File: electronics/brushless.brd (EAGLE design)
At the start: 35.5 x 43.3 mm, 69 parts, among them J1 USB_MINI-B_SMT, Q1 BUK7Y12-40E, Q2 BUK7Y12-40E, Q3 BUK7Y12-40E, Q4 BUK7Y12-40E, Q5 BUK7Y12-40E, Q6 BUK7Y12-40E, X1 JST-XH-10-PIN-LONG-PAD

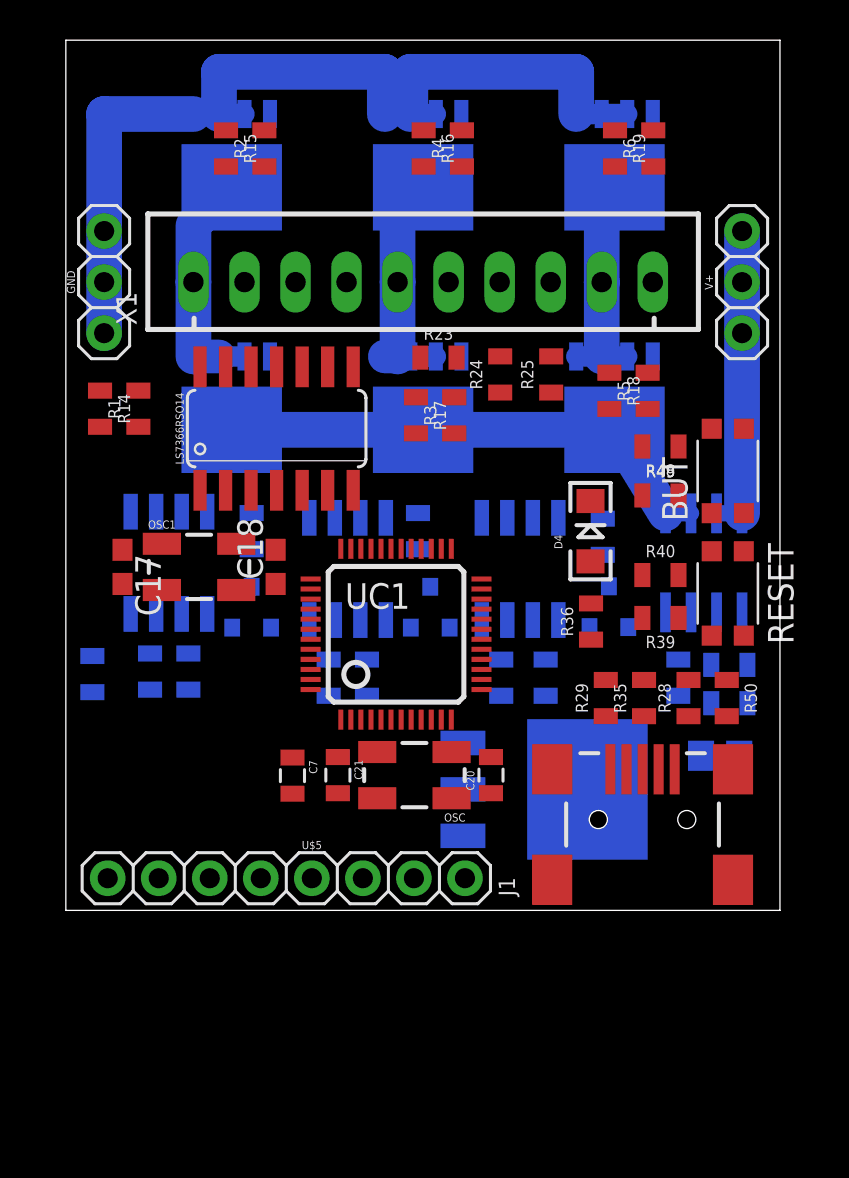
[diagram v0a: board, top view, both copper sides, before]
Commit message: Controller board
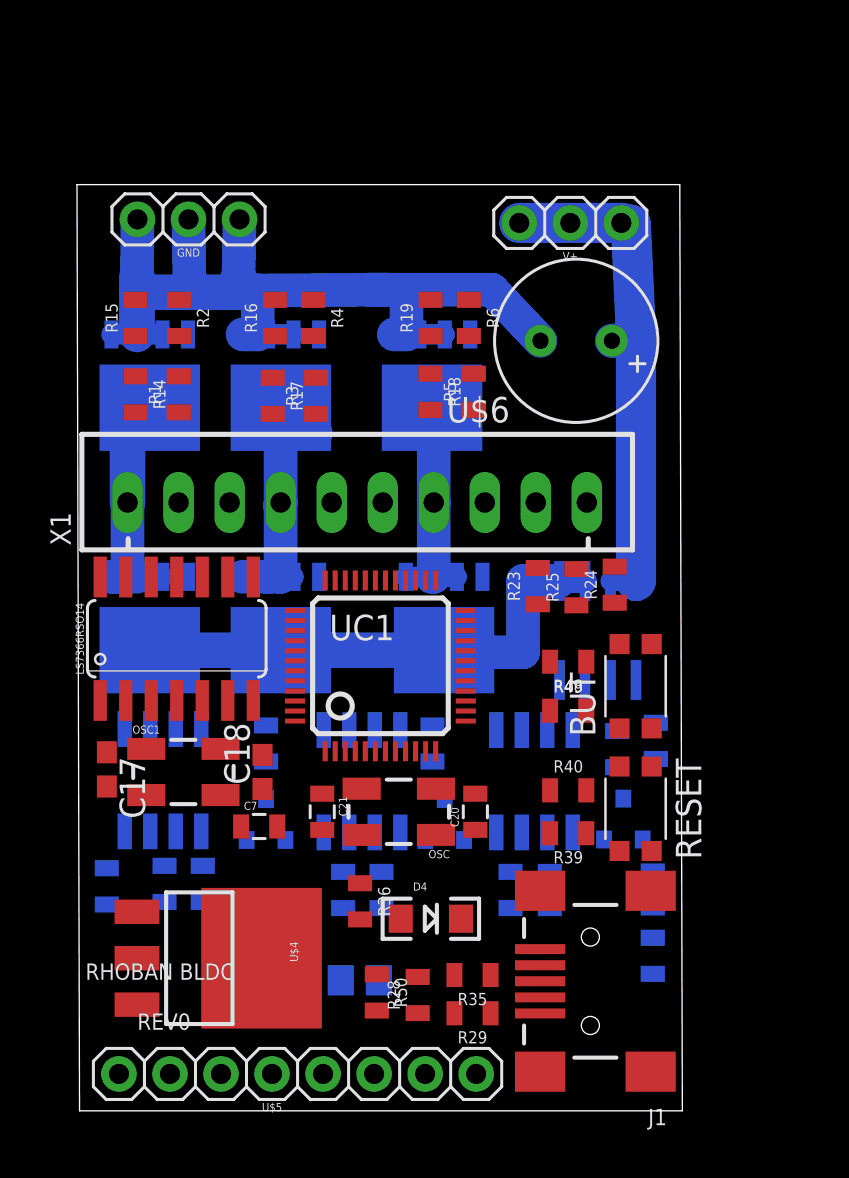
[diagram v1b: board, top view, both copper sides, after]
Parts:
- added U$6: (no value), rhoban:E3,5-8
- moved R50 22.8 mm to (14.8, 9.10)
- moved R13 21.1 mm to (14.0, 9.70), turned to 180 degrees
- moved D4 20.9 mm to (17.5, 12.8), turned to 0 degrees
- moved R28 20.0 mm to (16.9, 8.97)
- moved U$4 18.3 mm to (6.01, 10.8), flipped to the top, turned to 270 degrees
- moved R36 18.1 mm to (14.0, 13.6), turned to 270 degrees
- moved R29 17.0 mm to (19.6, 8.06), turned to 180 degrees
- moved R35 16.2 mm to (19.6, 9.97), turned to 180 degrees
- moved Q6 14.2 mm to (17.6, 39.2)
- moved Q5 13.9 mm to (18.2, 27.1)
- moved R21 13.1 mm to (28.6, 10.9), turned to 270 degrees
- moved Q3 13.1 mm to (10.1, 27.1)
- moved Q4 13.1 mm to (10.1, 39.2)
- moved R19 12.5 mm to (17.5, 42.7), turned to 90 degrees
- moved R6 12.5 mm to (19.4, 42.7), turned to 270 degrees
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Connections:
- net ENC_B: now also X1.5; no longer X1.4
- net GND: now also U$6.-
- net HALLV: now also X1.9; no longer X1.7
- net V+: now also U$6.+
- net V_PHASE: now also X1.4; no longer X1.5
- net W_PHASE: now also X1.7; no longer X1.9
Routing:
- net V+: track 15.3 -> 25.9 mm
- net V_PHASE: track 11.5 -> 14.4 mm
- net U_PHASE: track 14.4 -> 12.2 mm
- net GND: track 47.9 -> 49.4 mm
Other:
- board size 35.5 x 43.3 mm -> 30.1 x 46.1 mm
- board text added: "REV0"
- board text added: "RHOBAN BLDC"

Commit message: Small tweaks
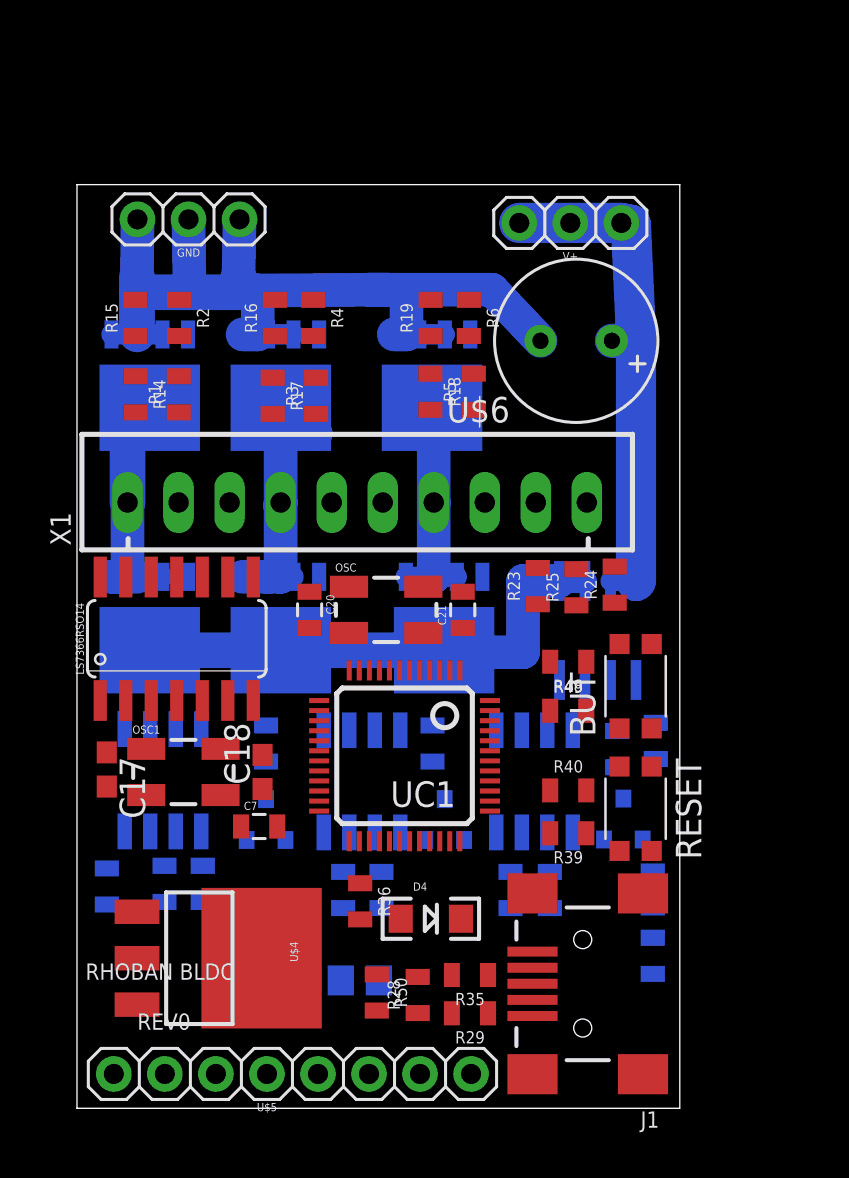
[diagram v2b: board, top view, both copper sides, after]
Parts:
- moved C20 13.0 mm to (11.5, 28.1), turned to 270 degrees
- moved C21 12.2 mm to (19.1, 28.1), turned to 90 degrees
- moved OSC 10.1 mm to (15.3, 28.1), turned to 0 degrees
- moved UC1 4.64 mm to (16.2, 20.9), turned to 180 degrees
- moved J1 0.40 mm to (25.1, 9.53)
- moved U$5 0.25 mm to (9.37, 5.04)
- moved R29 0.13 mm to (19.5, 8.06)
- moved R35 0.13 mm to (19.5, 9.97)
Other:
- board size 30.1 x 46.1 mm -> 30 x 46 mm
